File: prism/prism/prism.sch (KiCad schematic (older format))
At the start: 11 parts, among them J1 in1, J2 in2, J3 in3, J4 in4, J5 out1, J6 out2, J7 out3, J8 out4, SW1 Rotary_Encoder_Switch, U1 MCP4728

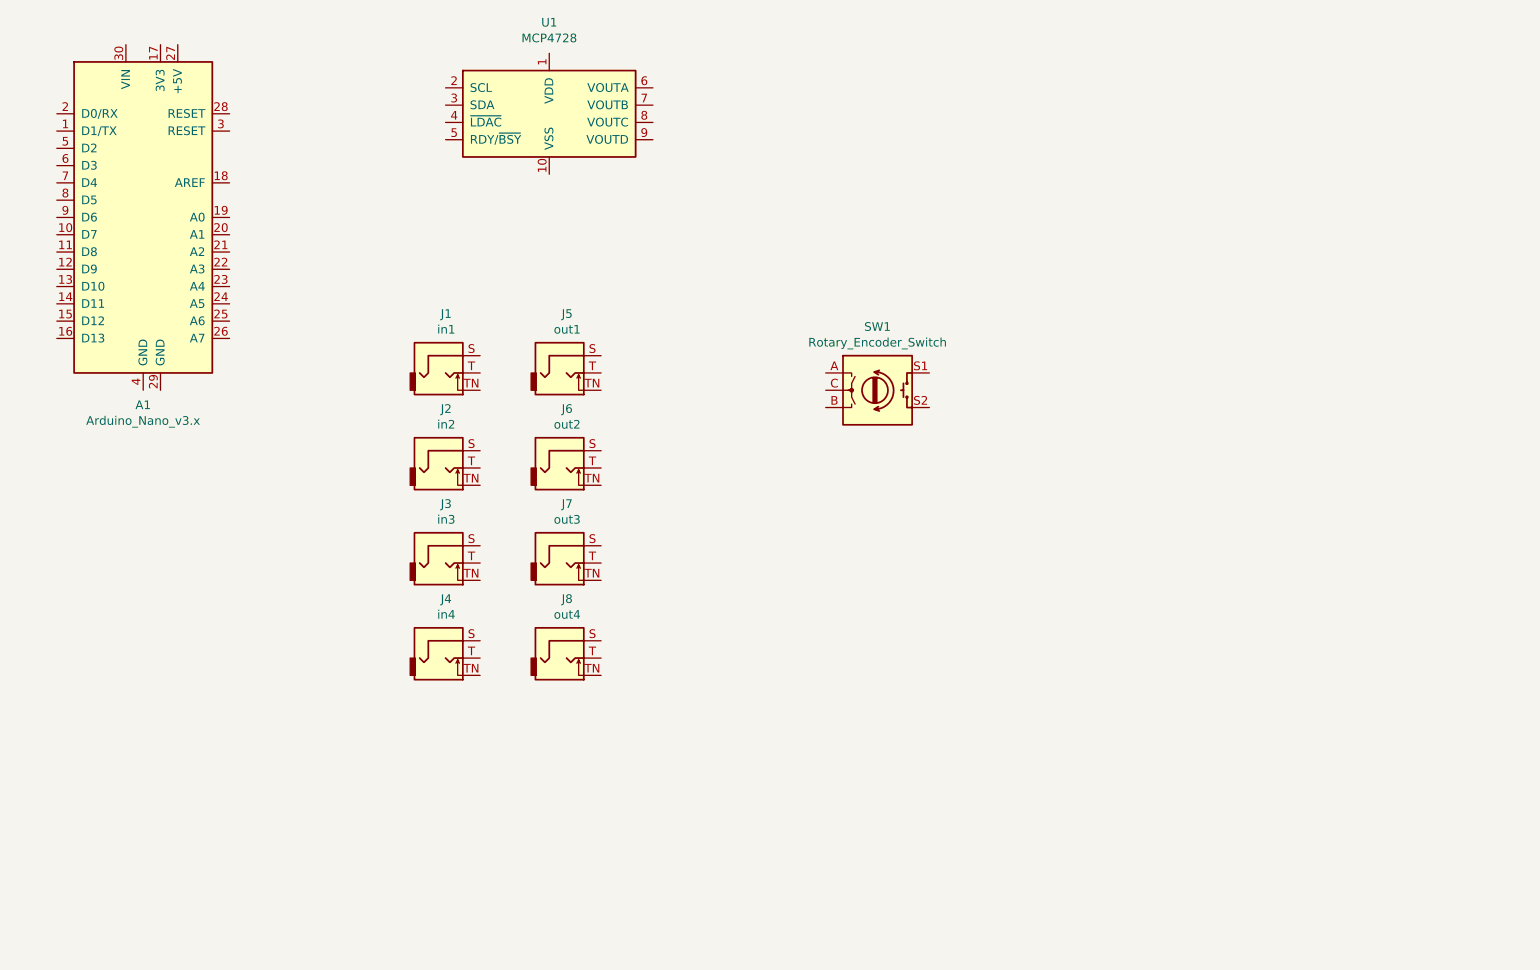
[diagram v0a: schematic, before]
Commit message: All kinds of stuff
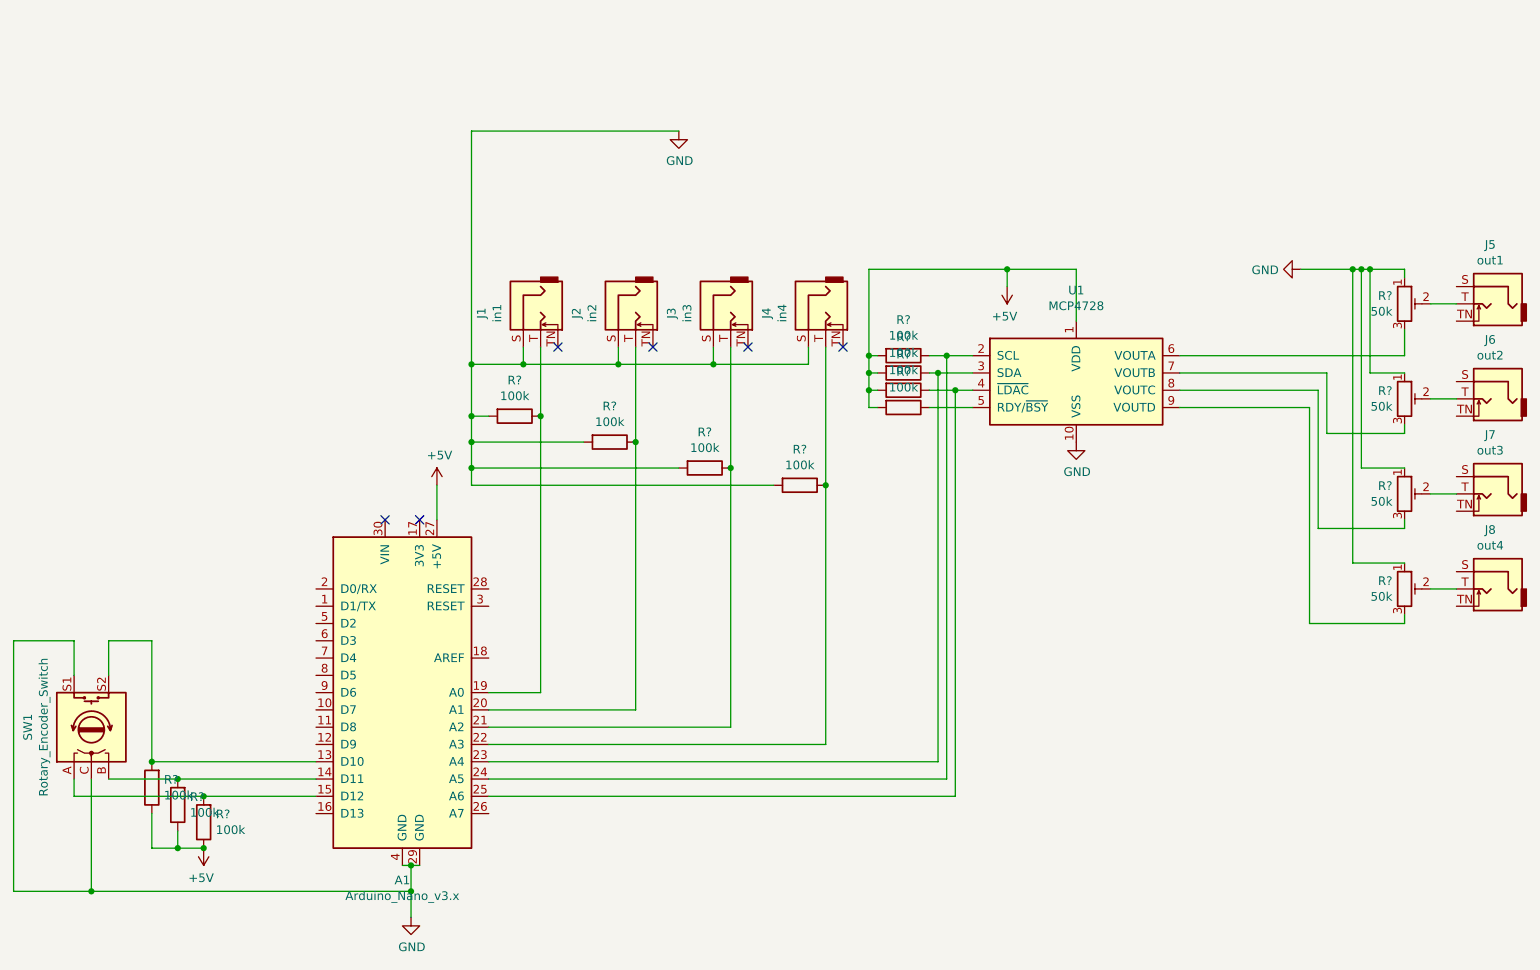
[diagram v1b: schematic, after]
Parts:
- added R? (x11): 100k, Resistor_THT:R_Axial_DIN0207_L6.3mm_D2.5mm_P7.62mm_Horizontal, symbol Device:R
- added R? (x4): 50k, Potentiometer_THT:Potentiometer_Bourns_3296W_Vertical, symbol Device:R_POT_TRIM
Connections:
- net at SW1.A: now also A1.15 (D12), R?.2
- net at SW1.B: now also A1.14 (D11), R?.2
- net GND: now reaches SW1.C
- net GND: now also A1.29 (GND), A1.4 (GND), J1.S, J2.S, J3.S, J4.S, SW1.S1, U1.10 (VSS), R?.1, R?.1, R?.1, R?.1, R?.2, R?.2, R?.2, R?.2
- net at SW1.S2: now also A1.13 (D10), R?.2
- net at J1.T: now also A1.19 (A0), R?.1
- net at J2.T: now also A1.20 (A1), R?.1
- net at J3.T: now also A1.21 (A2), R?.1
- net at J4.T: now also A1.22 (A3), R?.1
- net at J5.T: now also R?.2
- net at J6.T: now also R?.2
- net at J7.T: now also R?.2
- net at J8.T: now also R?.2
- net at A1.23 (A4): now also U1.3 (SDA), R?.1
- net at A1.24 (A5): now also U1.2 (SCL), R?.1
- net at A1.25 (A6): now also U1.4 (~LDAC), R?.1
- net +5V: now reaches A1.27 (+5V)
- net +5V: now also U1.1 (VDD), R?.1, R?.1, R?.1, R?.2, R?.2, R?.2, R?.2
- net at U1.5 (RDY/~BSY): now also R?.1
- net at U1.6 (VOUTA): now also R?.3
- net at U1.7 (VOUTB): now also R?.3
- net at U1.8 (VOUTC): now also R?.3
- net at U1.9 (VOUTD): now also R?.3
- no-connect marks 0 -> 6
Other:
- moved on the sheet: A1, J1, J2, J3, J4, J5, J6, J7, J8, SW1, U1
